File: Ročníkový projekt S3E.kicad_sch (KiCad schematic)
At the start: 39 parts, among them IC1 PIC18F47Q43-I_P, IC3 ULN2804A, IC5 MCP7940M-I_SN, J1 DG126-5.0-02P-14-00A, J2 - nastavení času, J3 + nastavení času, J7 TSW-105-07-G-S, J8 přepínání mezi číslicemi, Q1 DTA123JCAT116, Q2 DTA123JCAT116, Q3 DTA123JCAT116, Q4 DTA123JCAT116, Q5 DTA123JCAT116, Q6 DTA123JCAT116, Y1 32.768kHz

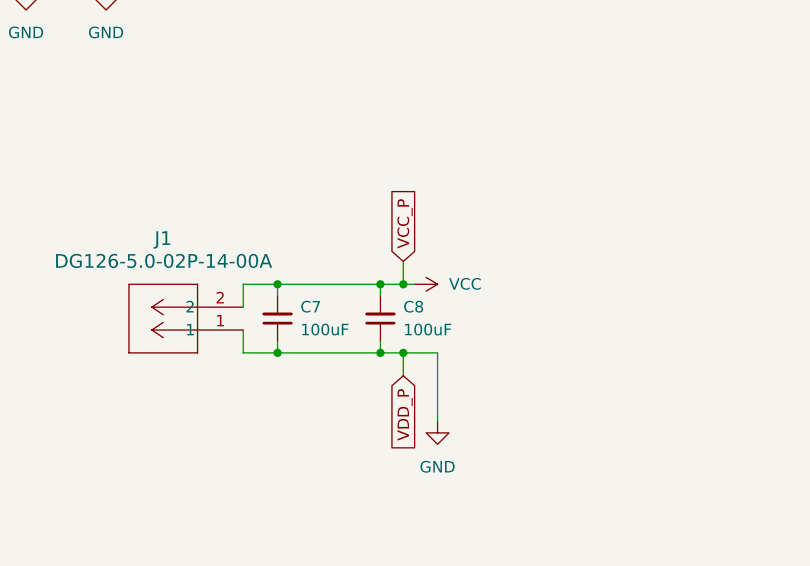
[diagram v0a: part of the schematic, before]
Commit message: backup update
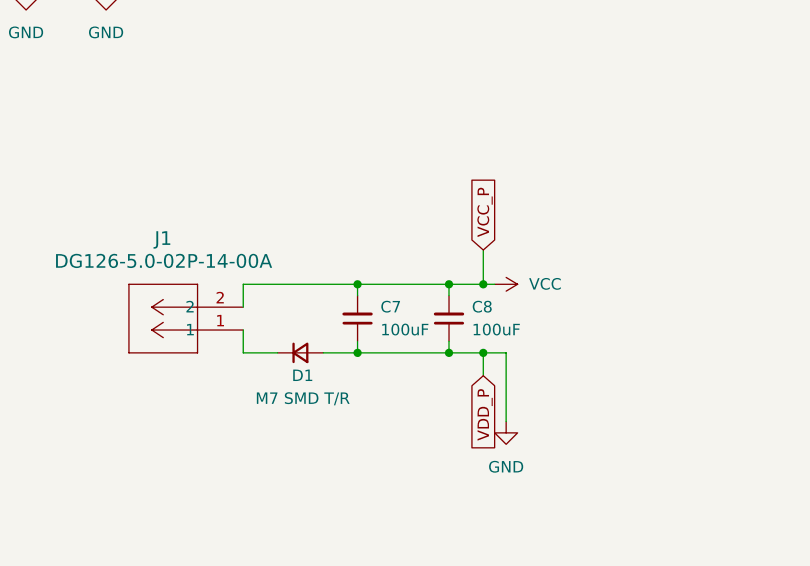
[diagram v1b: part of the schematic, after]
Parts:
- added D1: M7 SMD T/R, Diode_SMD:D_SMA_Handsoldering, symbol Device:D_Small
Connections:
- net GND: now also D1.2 (A); no longer J1.1
- new net: D1.1 (K), J1.1
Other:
- moved on the sheet: C7, C8
